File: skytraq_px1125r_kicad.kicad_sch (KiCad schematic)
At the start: 11 parts, among them J1 Conn_01x04, J2 SMA, J3 SH_Conn_01x04, J4 Conn_01x04, U1 Skytraq_PX1125R

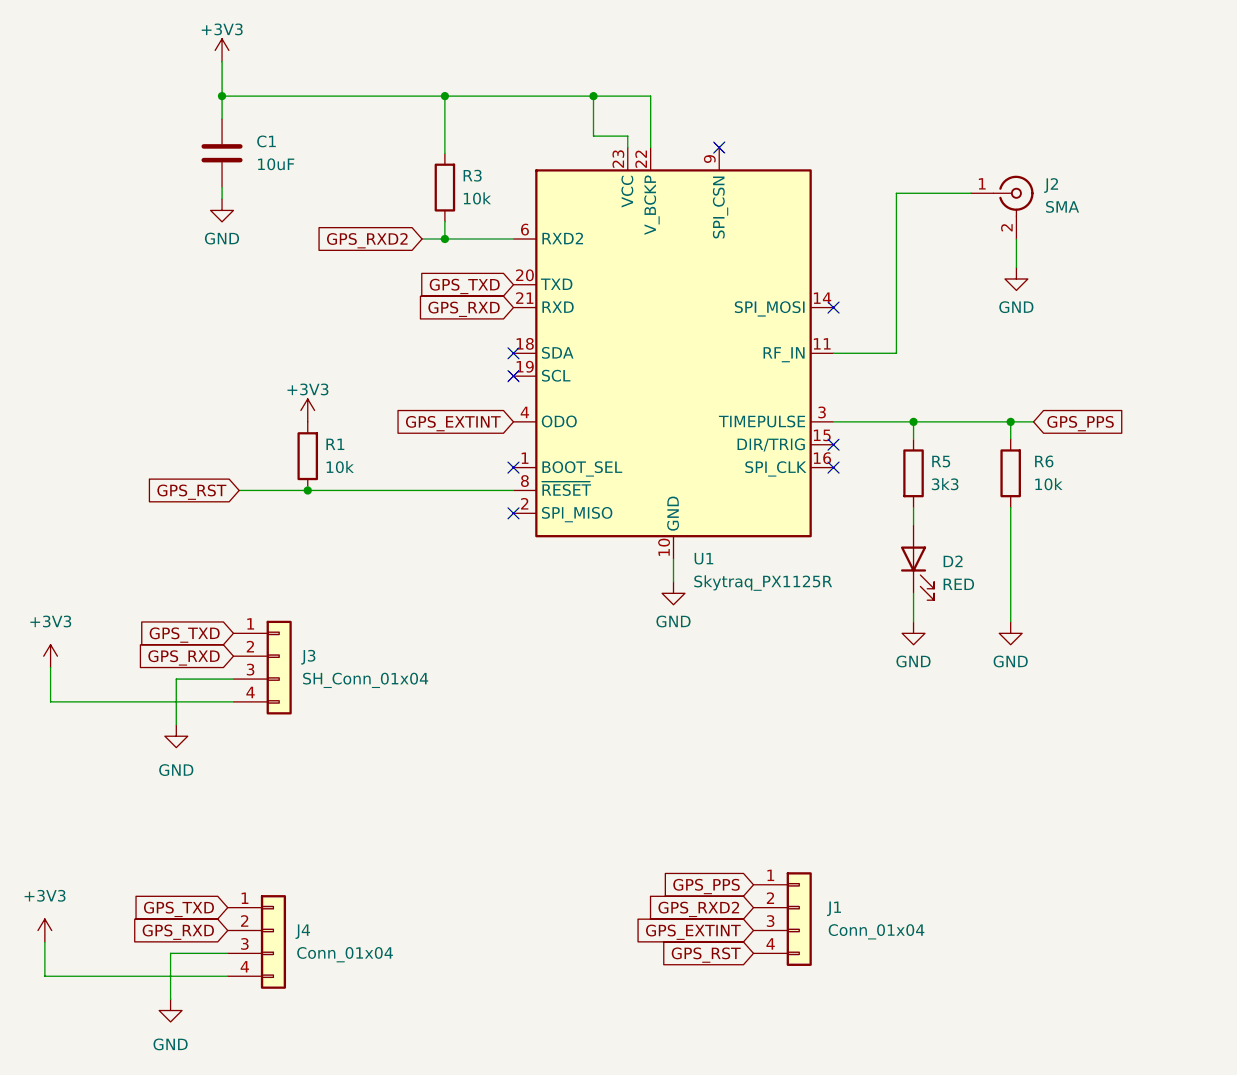
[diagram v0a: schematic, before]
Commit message: PX1105
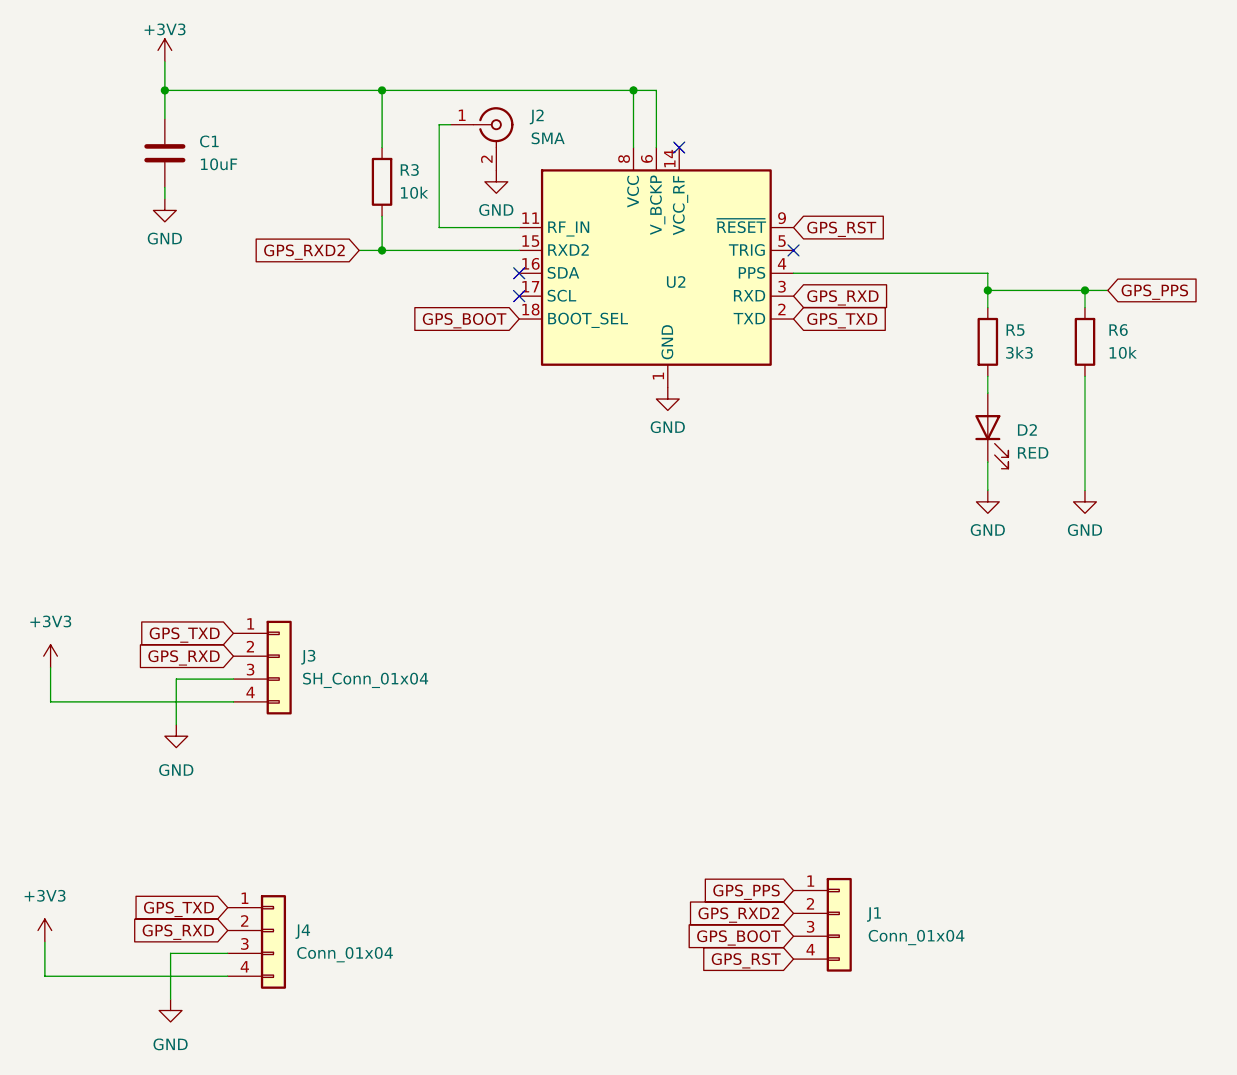
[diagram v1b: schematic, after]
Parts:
- removed R1: 10k, Resistor_SMD:R_0805_2012Metric_Pad1.20x1.40mm_HandSolder, symbol Device:R
- removed U1: Skytraq_PX1125R, RF_GPS:ublox_NEO, symbol MySymbols:Skytraq_PX1125R
- added U2: ~, MySkyTraqFootprints:skytraq_px1105, symbol MySkyTraqSymbols:SkyTraq_PX1105
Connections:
- net +3V3: now also U2.6 (V_BCKP), U2.8 (VCC)
- net GND: now also U2.1 (GND)
- net GPS_PPS: now also U2.4 (PPS)
- net GPS_RST: now also U2.9 (~{RESET})
- net GPS_RXD: now also U2.3 (RXD)
- net GPS_RXD2: now also U2.15 (RXD2)
- net GPS_TXD: now also U2.2 (TXD)
- net at J2.1 (In): now also U2.11 (RF_IN)
- net GPS_EXTINT renamed GPS_BOOT
- net GPS_BOOT: now also U2.18 (BOOT_SEL)
- no-connect marks 8 -> 4
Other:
- moved on the sheet: C1, D2, J1, J2, R3, R5, R6
